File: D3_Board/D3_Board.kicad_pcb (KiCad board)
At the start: 2 copper layers, 115 x 83 mm, 46 parts, among them J1 POWER_IN, J10 ACS_SENSOR, J11 H-BRIDGE1, J12 H-BRIDGE2, J13 BUZZER, J14 MOTOR1_POW, J15 MOTOR1_OUT, J16 MOTOR2_POW, J17 MOTOR2_OUT, J2 POWER_IN, J3 RASPBERRY_POWER_IN, J4 RASPBERRY, J5 CURRENT_POWER_IN, J6 LED_Matrix, J7 USB_TTL, J8 MOTOR1, J9 MOTOR2, M1 SERVO2, M2 SERVO1, Q1 BC546, Q2 BC546, Q3 BC546, Q4 BC546, U1 Bluepill, U2 LM2596, U3 GPS_NEO6M, U4 MPU6050

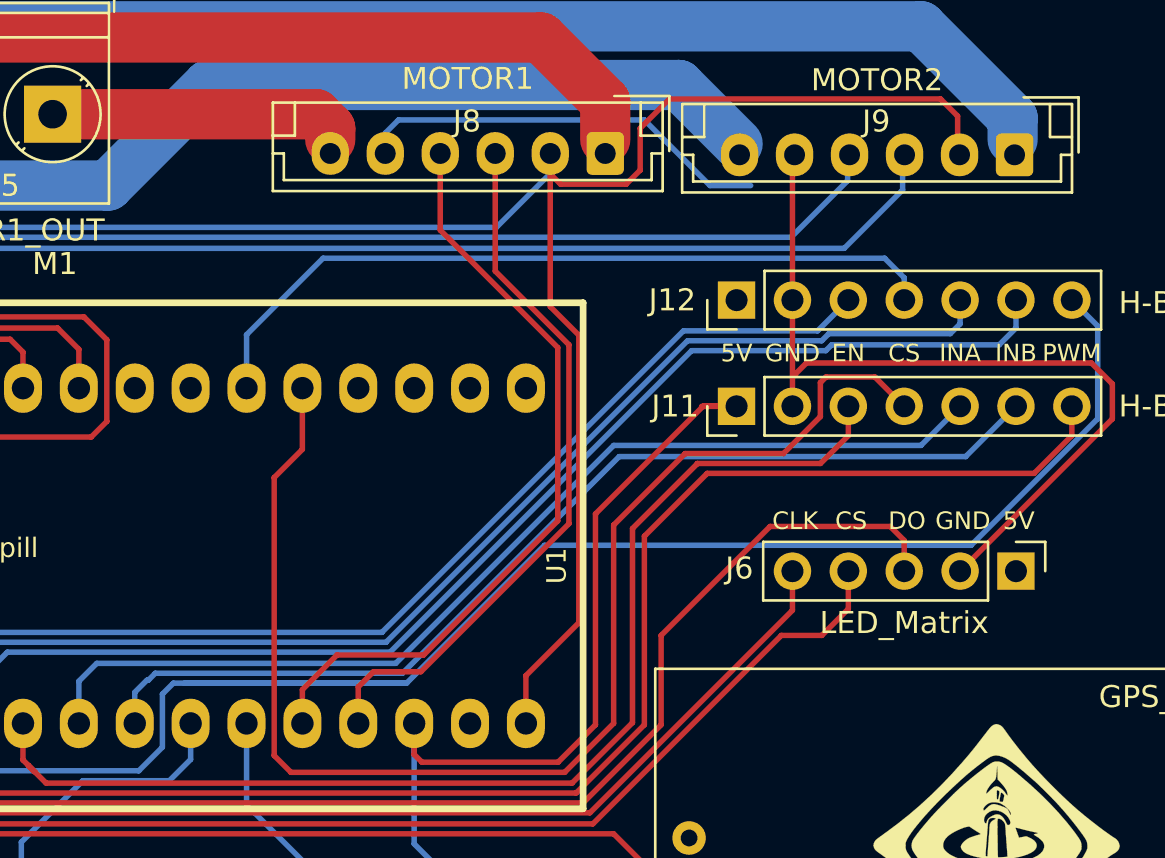
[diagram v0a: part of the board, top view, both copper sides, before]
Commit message: Update main board Schematics
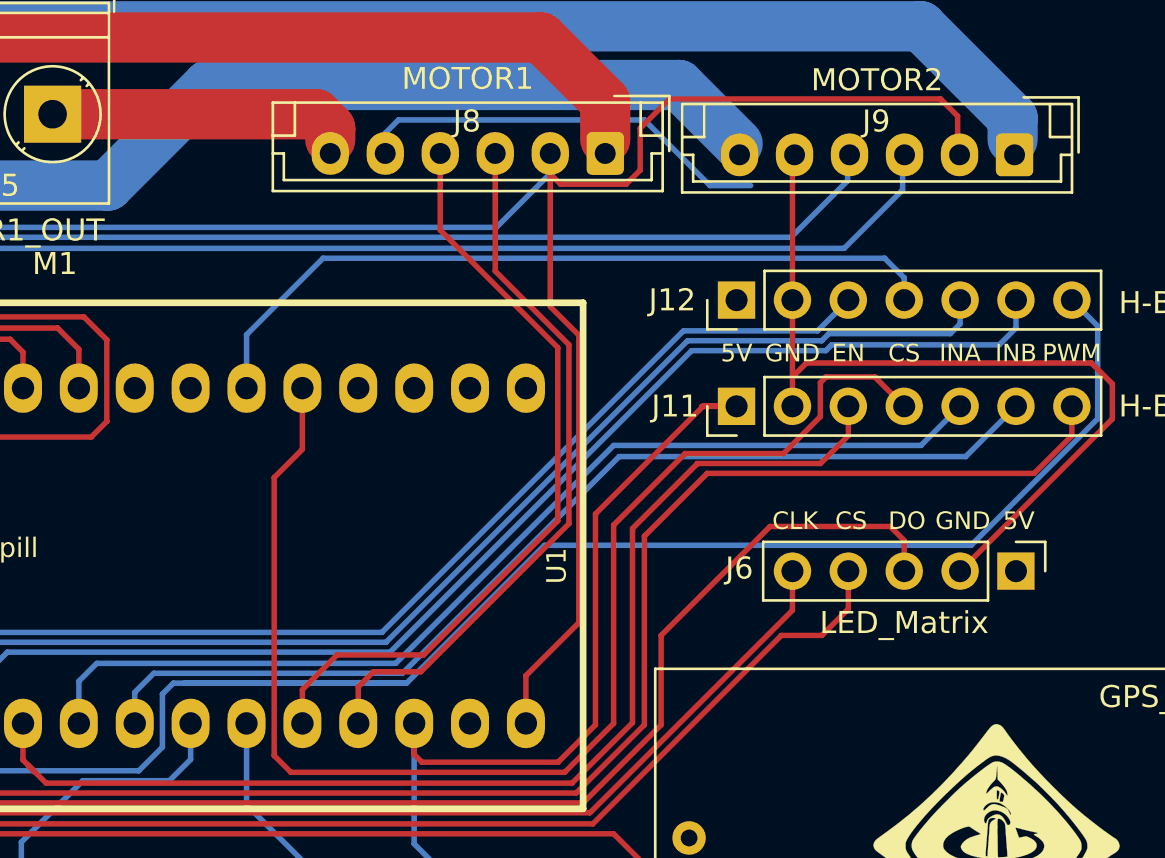
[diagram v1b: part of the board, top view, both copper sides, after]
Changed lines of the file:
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@@
-(kicad_pcb (version 20171130) (host pcbnew 5.1.9-73d0e3b20d~88~ubuntu20.04.1)
+(kicad_pcb (version 20171130) (host pcbnew 5.1.10-88a1d61d58~88~ubuntu20.04.1)
   (general
     (thickness 1.6)
     (drawings 49)
-    (tracks 352)
+    (tracks 350)
     (zones 0)
     (modules 46)
@@
   (page A4)
   (layers
-    (0 F.Cu signal hide)
-    (31 B.Cu signal hide)
+    (0 F.Cu signal)
+    (31 B.Cu signal)
     (32 B.Adhes user)
     (33 F.Adhes user)
@@
     (visible_elements FFFFFF7F)
     (pcbplotparams
-      (layerselection 0x010fc_ffffffff)
-      (usegerberextensions false)
+      (layerselection 0x010f0_ffffffff)
+      (usegerberextensions true)
       (usegerberattributes true)
       (usegerberadvancedattributes true)
@@
       (psnegative false)
       (psa4output false)
-      (plotreference true)
+      (plotreference false)
       (plotvalue true)
       (plotinvisibletext false)
@@
       (outputformat 1)
       (mirror false)
-      (drillshape 1)
+      (drillshape 0)
       (scaleselection 1)
-      (outputdirectory ""))
+      (outputdirectory "gerbers/"))
   )
   (net 0 "")
@@
     (pad 2 thru_hole oval (at 2.5 0 180) (size 1.7 1.95) (drill 0.95) (layers *.Cu *.Mask)
       (net 14 +3V3))
-    (pad 1 thru_hole roundrect (at 0 0 180) (size 1.7 1.95) (drill 0.95) (layers *.Cu *.Mask) (roundrect_rratio 0.147059)
+    (pad 1 thru_hole roundrect (at 0 0 180) (size 1.7 1.95) (drill 0.95) (layers *.Cu *.Mask) (roundrect_rratio 0.1470588235294118)
       (net 21 /MOTOR2_M2))
     (model ${KISYS3DMOD}/Connector_JST.3dshapes/JST_EH_B6B-EH-A_1x06_P2.50mm_Vertical.wrl
@@
     (pad 2 thru_hole oval (at 2.5 0 180) (size 1.7 1.95) (drill 0.95) (layers *.Cu *.Mask)
       (net 14 +3V3))
-    (pad 1 thru_hole roundrect (at 0 0 180) (size 1.7 1.95) (drill 0.95) (layers *.Cu *.Mask) (roundrect_rratio 0.147059)
+    (pad 1 thru_hole roundrect (at 0 0 180) (size 1.7 1.95) (drill 0.95) (layers *.Cu *.Mask) (roundrect_rratio 0.1470588235294118)
       (net 13 /MOTOR1_M2))
     (model ${KISYS3DMOD}/Connector_JST.3dshapes/JST_EH_B6B-EH-A_1x06_P2.50mm_Vertical.wrl
@@
   (segment (start 34.4932 35.31447) (end 35.93421 36.75548) (width 0.25) (layer F.Cu) (net 22))
   (segment (start 34.4932 33.5915) (end 34.4932 35.31447) (width 0.25) (layer F.Cu) (net 22))
-  (segment (start 97.663 21.463) (end 99.949 19.177) (width 0.25) (layer B.Cu) (net 23))
-  (segment (start 81.915 21.463) (end 97.663 21.463) (width 0.25) (layer B.Cu) (net 23))
-  (segment (start 72.06699 31.31101) (end 81.915 21.463) (width 0.25) (layer B.Cu) (net 23))
-  (segment (start 60.82749 31.31101) (end 72.06699 31.31101) (width 0.25) (layer B.Cu) (net 23))
-  (segment (start 60.5155 31.623) (end 60.82749 31.31101) (width 0.25) (layer B.Cu) (net 23))
-  (segment (start 60.452 31.623) (end 60.5155 31.623) (width 0.25) (layer B.Cu) (net 23))
-  (segment (start 59.8932 32.1818) (end 60.452 31.623) (width 0.25) (layer B.Cu) (net 23))
-  (segment (start 59.8932 33.5915) (end 59.8932 32.1818) (width 0.25) (layer B.Cu) (net 23))
+  (segment (start 60.76399 31.31101) (end 59.8932 32.1818) (width 0.25) (layer B.Cu) (net 23))
+  (segment (start 72.06699 31.31101) (end 60.76399 31.31101) (width 0.25) (layer B.Cu) (net 23))
+  (segment (start 59.8932 32.1818) (end 59.8932 33.5915) (width 0.25) (layer B.Cu) (net 23))
+  (segment (start 81.915 21.463) (end 72.06699 31.31101) (width 0.25) (layer B.Cu) (net 23))
+  (segment (start 97.663 21.463) (end 81.915 21.463) (width 0.25) (layer B.Cu) (net 23))
+  (segment (start 99.949 19.177) (end 97.663 21.463) (width 0.25) (layer B.Cu) (net 23))
   (segment (start 97.409 19.177) (end 95.631 20.955) (width 0.25) (layer B.Cu) (net 24))
   (segment (start 71.755 30.861) (end 81.661 20.955) (width 0.25) (layer B.Cu) (net 24))
